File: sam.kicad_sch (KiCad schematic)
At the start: 47 parts, among them IC11 74ACT244N, IC16 74ACT244N, IC31 74ACT02, IC33 74ACT138N, J4 JTAG, U1 74ACT138, U1 AS6C1008-TIN, U2 AS6C1008-55TIN, U3 XC95144XL-TQ100, U4 TPS7A2433DBVR, X1 14.31818MHz

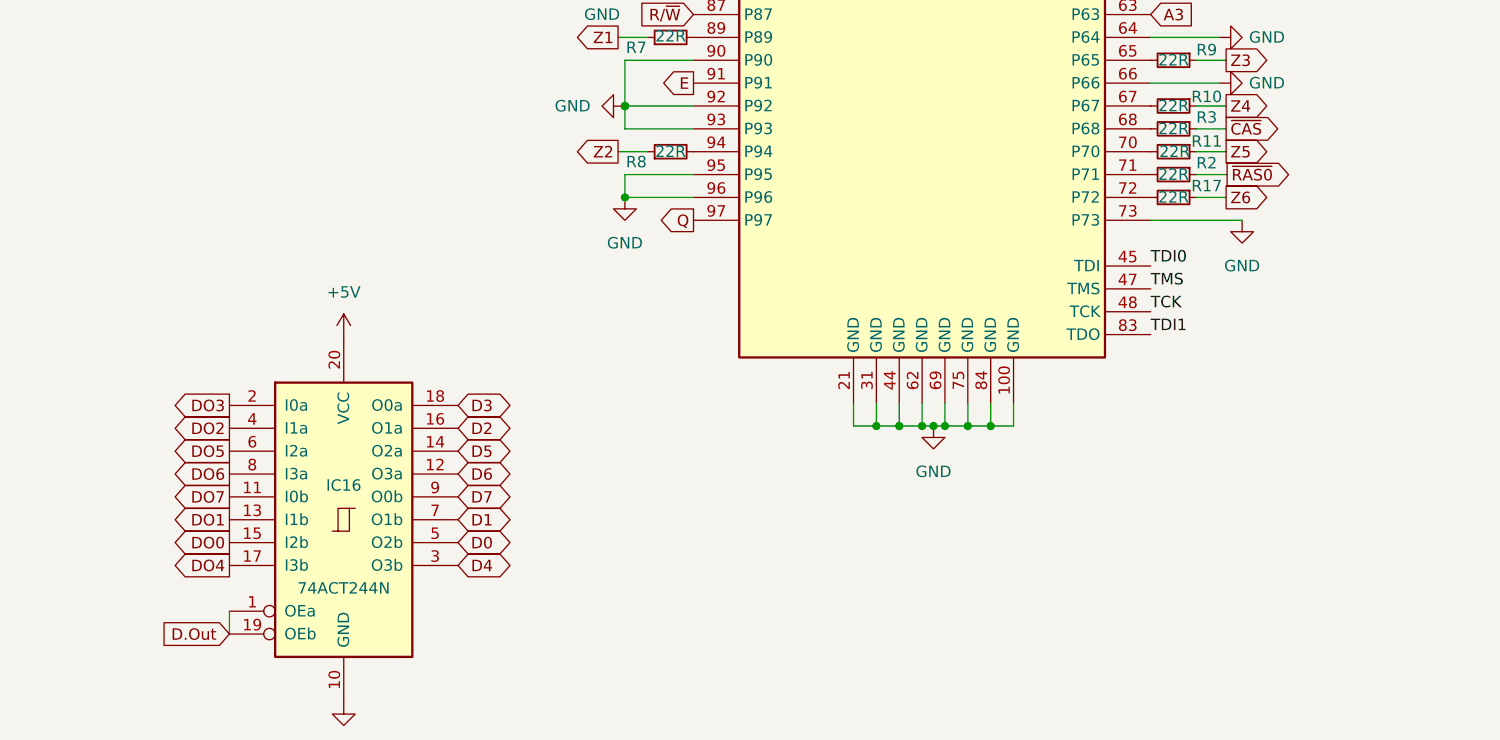
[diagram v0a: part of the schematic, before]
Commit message: serial wiring
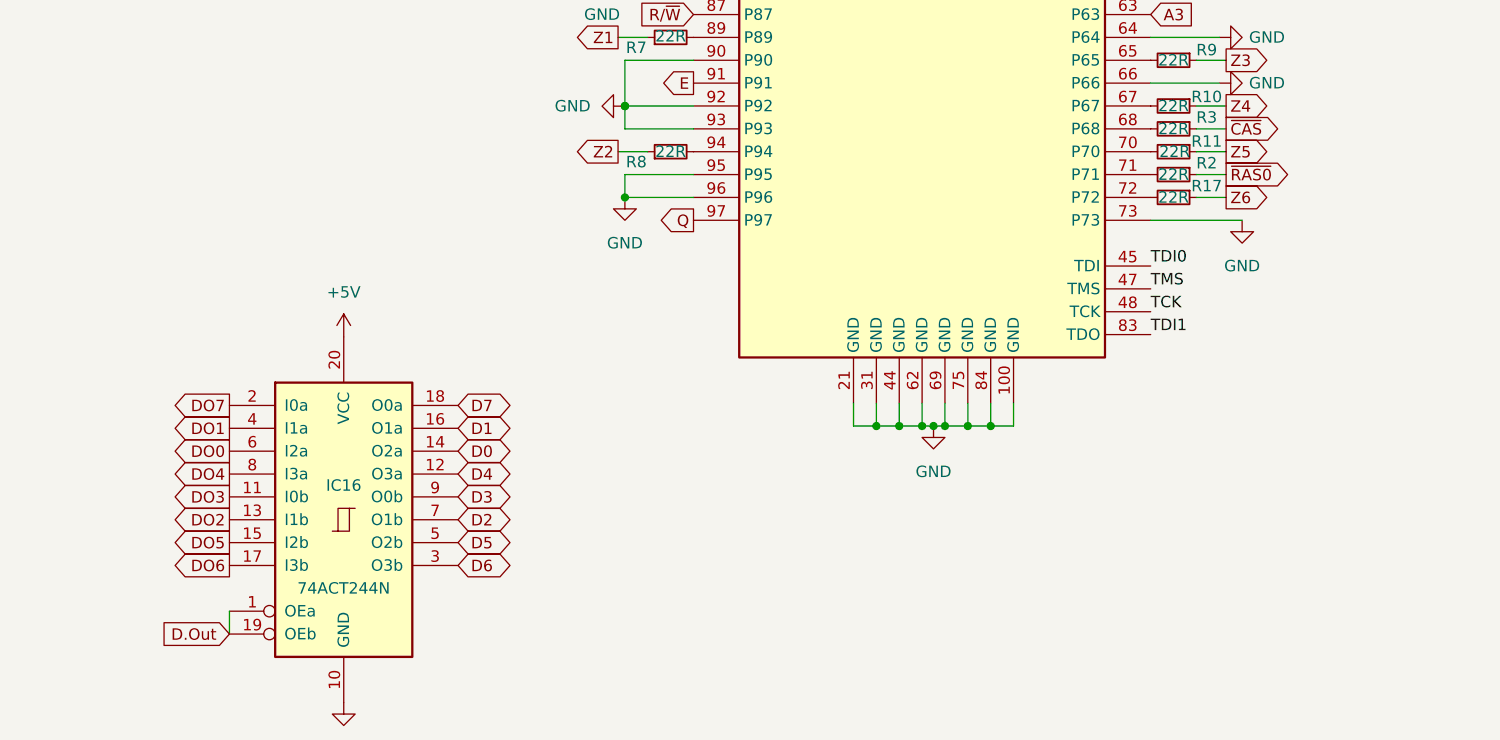
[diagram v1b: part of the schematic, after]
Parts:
- IC33, U1: footprint Package_SO:SOIC-20W_7.5x12.8mm_P1.27mm -> Package_SO:SOIC-16W_7.5x10.3mm_P1.27mm
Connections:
- net D0: now also IC16.14 (O2a); no longer IC16.5 (O2b)
- net D1: now also IC16.16 (O1a); no longer IC16.7 (O1b)
- net D2: now also IC16.7 (O1b); no longer IC16.16 (O1a)
- net D3: now also IC16.9 (O0b); no longer IC16.18 (O0a)
- net D4: now also IC16.12 (O3a); no longer IC16.3 (O3b)
- net D5: now also IC16.5 (O2b); no longer IC16.14 (O2a)
- net D6: now also IC16.3 (O3b); no longer IC16.12 (O3a)
- net D7: now also IC16.18 (O0a); no longer IC16.9 (O0b)
- net DO0: now also IC16.6 (I2a); no longer IC16.15 (I2b)
- net DO1: now also IC16.4 (I1a); no longer IC16.13 (I1b)
- net DO2: now also IC16.13 (I1b); no longer IC16.4 (I1a)
- net DO3: now also IC16.11 (I0b); no longer IC16.2 (I0a)
- net DO4: now also IC16.8 (I3a); no longer IC16.17 (I3b)
- net DO5: now also IC16.15 (I2b); no longer IC16.6 (I2a)
- net DO6: now also IC16.17 (I3b); no longer IC16.8 (I3a)
- net DO7: now also IC16.2 (I0a); no longer IC16.11 (I0b)
- net ~{RAS0}: now also R2.1
